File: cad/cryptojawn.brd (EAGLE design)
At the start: 45.5 x 15 mm, 36 parts, among them CN1 MICROSDPLAIN, CN2 HEADER-3X2-PTH1.27, Q1 IRLML6344TRPBF, SW1 SWITCHKMR211, SW2 SWITCHKMR211, U1 STM32F4/64, U2 EEPROM-I2C-8-DFN8W, X1 12MHz, X2 USB-A

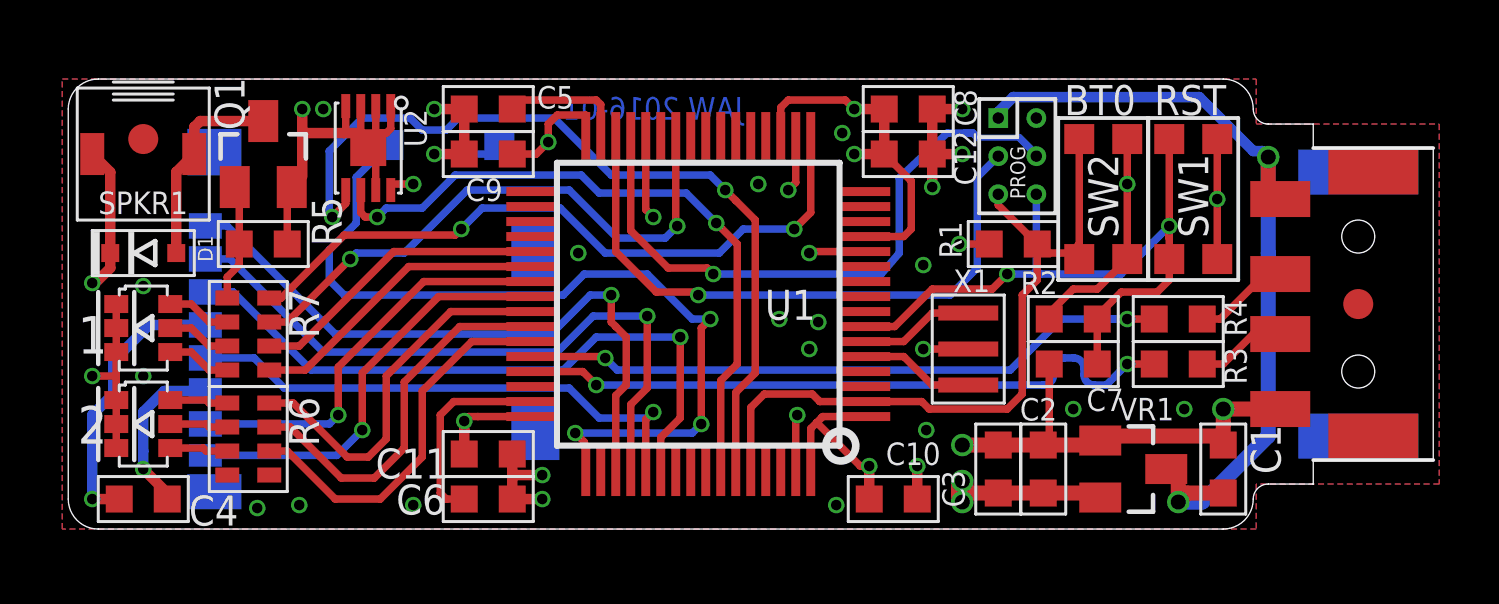
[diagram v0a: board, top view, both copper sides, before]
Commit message: hardware rev.1
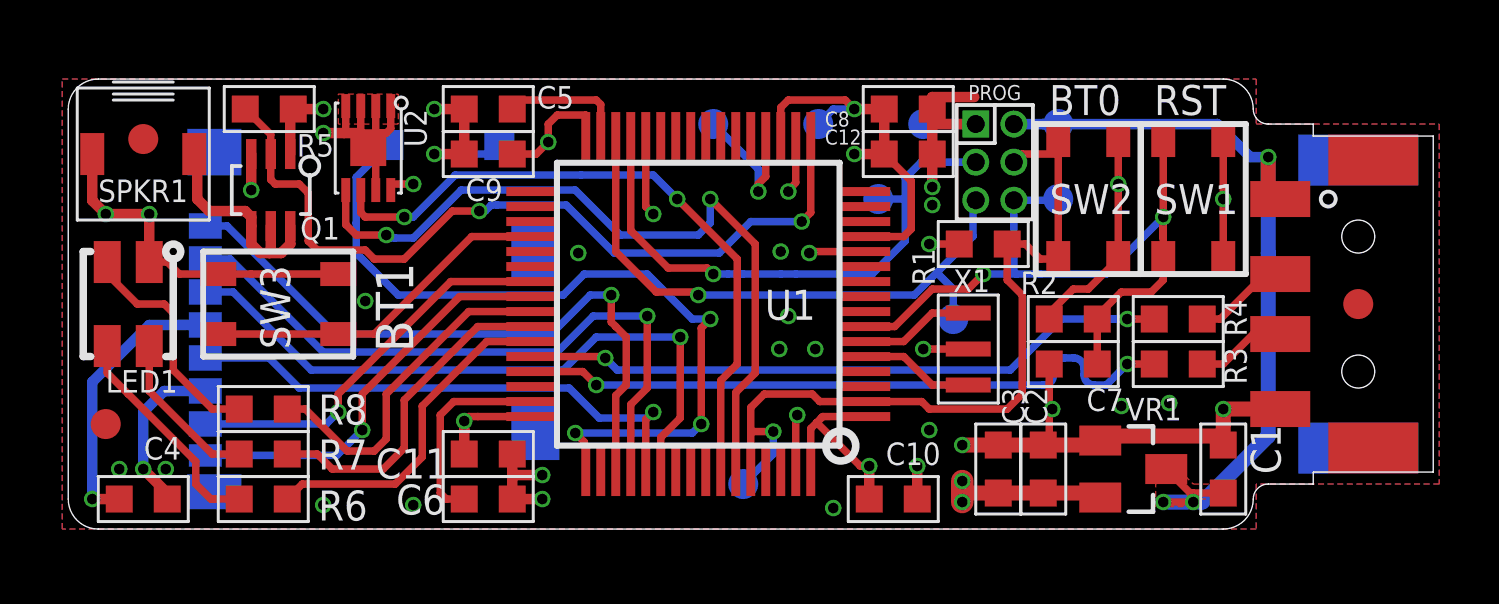
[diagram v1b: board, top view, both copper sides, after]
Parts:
- removed D1: any, jaw:SOD-323
- removed LED2: LED_RGB3, jaw:SMDLEDRGB
- removed X2: USB-A, jaw:MOLEX_480371000
- added CN10, CN11, CN4, CN5, CN6, CN7, CN8, CN9: HEADER-1X1-SPOT, jaw-conn:SPOT
- added CN3: USB-A-2100, jaw-conn:MOLEX_480372100
- added R8: 470, jaw:SMD0603
- added SW3: SWITCH-PTS810, jaw:PTS810
- added U$4: FIDUCIAL, adafruit:FIDUCIAL_1MM
- CN2: value HEADER-3X2-PTH1.27 -> DO NOT PLACE; device jaw:HEADER-3X2-PTH1.27 -> jaw-conn:HEADER-3X2-PTH1.27
- LED1: value LED_RGB3 -> LED-RGB-CA-PLCC4; device jaw:SMDLEDRGB -> jaw:PLCC4-3228
- Q1: value IRLML6344TRPBF -> MOSFET-2N; device jaw:SOT-23 -> jaw:SC-70-6
- R6, R7: device jaw:SMD-0603-ARV -> jaw:SMD0603
- SW1, SW2: value SWITCHKMR211 -> SWITCH-PTS810; device jaw:KMR211 -> jaw:PTS810
- VR1: device jaw:SOT-23-3 -> jaw:SOT-23-3@1
- moved U$1 5.70 mm to (34.8, 14.5)
- moved R5 4.50 mm to (17.2, 24.0)
- moved R7 4.03 mm to (17.0, 12.5), turned to 180 degrees
- moved R6 2.06 mm to (17.0, 11.0), turned to 180 degrees
- moved Q1 1.23 mm to (17.2, 21.3), turned to 270 degrees
- moved R1 1.00 mm to (41.0, 19.5)
- moved LED1 0.94 mm to (12.5, 17.5), turned to 270 degrees
- moved CN2 0.78 mm to (40.8, 23.5)
- moved SW2 0.50 mm to (44.5, 21.0), turned to 180 degrees
- turned SW1 to 180 degrees
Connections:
- removed net N$10: LED2.AB, R6.5
- removed net N$6: LED2.AR, R6.6
- removed net N$9: Q1.1, R5.1, R7.5
- new net IOTEST: CN11.P$1, U1.20
- net BOOT0: now also CN2.4, CN8.P$1, SW2.P$2, SW2.P$2B; no longer CN2.5, SW2.2, SW2.4
- net GND: now also CN2.1, CN3.4, CN3.P$1, CN3.P$2, CN3.P$3, CN3.P$4, CN5.P$1, Q1.1, SW1.P$1, SW1.P$1B; no longer CN2.2, LED1.CB, LED1.CG, LED1.CR, LED2.CB, LED2.CG, LED2.CR, Q1.2, SW1.1, SW1.3, X2.4
- net IOLED0: now also R6.1; no longer R6.2
- net IOLED1: now also R7.1; no longer R6.3
- net IOLED2: now also R8.1; no longer R6.4
- net IOLED3: no longer R7.1
- net IOLED4: no longer R7.2
- net IOLED5: no longer R7.3
- net IOSPKR: now also Q1.2, R5.1; no longer R7.4
- net N$1: now also LED1.P$4, R7.2; no longer LED1.AG, R7.8
- net N$14: now also Q1.4, Q1.5, Q1.6; no longer D1.A, Q1.3
- net N$2: now also SW3.P$1, SW3.P$1B, U1.36; no longer LED1.AR, R7.7
- net N$3: now also LED1.P$2, R8.2; no longer LED1.AB, R7.6
- net N$5: now also LED1.P$3, R6.2; no longer LED2.AG, R6.7
- net N$7: now also CN3.2; no longer X2.2
- net N$8: now also CN3.3; no longer X2.3
- net NRST: now also CN9.P$1, SW1.P$2, SW1.P$2B; no longer SW1.2, SW1.4
- net RX: now also CN2.5, CN7.P$1; no longer CN2.3
- net TX: now also CN2.3, CN6.P$1; no longer CN2.4
- net VCC: now also CN10.P$1, LED1.P$1, Q1.3, SW2.P$1, SW2.P$1B, SW3.P$2, SW3.P$2B; no longer D1.C, SW2.1, SW2.3
- net VUSB: now also CN2.2, CN3.1, CN4.P$1; no longer CN2.1, X2.1
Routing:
- net IOLED5: track 19.3 -> 0.00 mm, vias 2 -> 0
- net IOLED3: track 10.1 -> 0.00 mm
- net IOLED4: track 10.0 -> 0.00 mm
- net N$2: track 2.15 -> 11.7 mm
- net VCC: track 54.4 -> 63.7 mm, vias 11 -> 13
- net N$3: track 2.15 -> 7.78 mm
- net N$5: track 1.94 -> 7.48 mm
- net GND: track 70.4 -> 65.4 mm, vias 37 -> 34
- net IOTEST: track 0.00 -> 4.82 mm, vias 0 -> 1
- net IOSPKR: track 23.0 -> 27.3 mm
- net N$9: track 3.93 -> 0.00 mm
- net N$1: track 2.15 -> 5.37 mm
- net I2CDA: track 28.4 -> 25.7 mm
- net TX: track 21.6 -> 18.9 mm
- net BOOT0: track 25.4 -> 27.4 mm, vias 0 -> 1
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- added copper zone on layer 1, net N$6
- added copper zone on layer 1, net VUSB
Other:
- outline, holes or cut-outs redrawn
- board text added: "BT1"
- board text added: "Designed in Philly, built by robots"
- board text added: "JAW 2018-08"
- board text added: "SD Card"
- board text added: "cryptojawn v1"
- board text removed: "1"
- board text removed: "2"
- board text removed: "JAW 2016-01"
- board text removed: "usb415 Rev. 1"
